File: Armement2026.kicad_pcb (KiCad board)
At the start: 2 copper layers, 87.5 x 61.5 mm, 24 parts, among them J1 Screw_Terminal_01x02, J10 Screw_Terminal_01x02, J11 Screw_Terminal_01x02, J12 Screw_Terminal_01x02, J2 Screw_Terminal_01x02, J5 Screw_Terminal_01x02, J6 Screw_Terminal_01x02, J8 Screw_Terminal_01x02, J9 Screw_Terminal_01x02, Q1 NTR4101PT1G, Q2 NTR4101PT1G, SW1 SW_Nidec_CAS-120A1, SW2 SW_Nidec_CAS-120A1, SW3 SW_Nidec_CAS-120A1, U1 LDO_4v2-MIC5209-4.2YS-TR

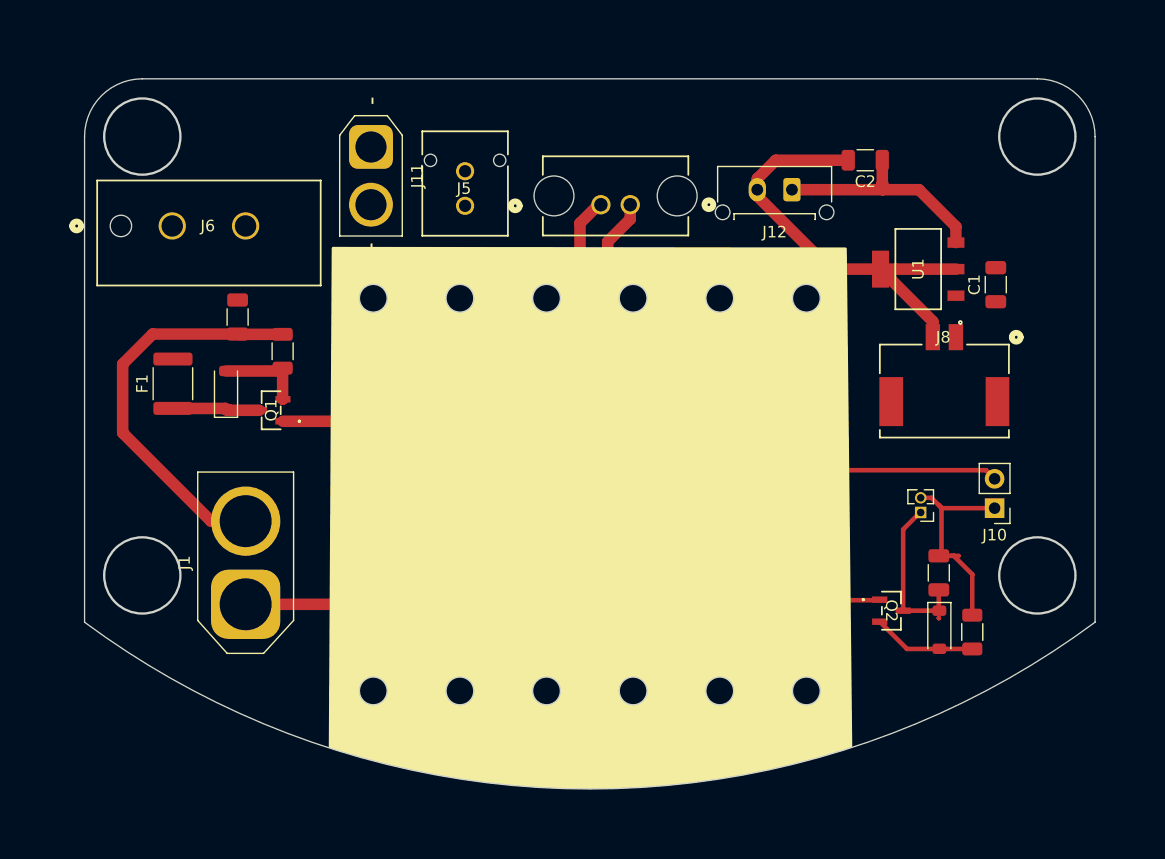
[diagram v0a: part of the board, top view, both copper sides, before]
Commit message: PCB Armement IRECxFAR-OUT
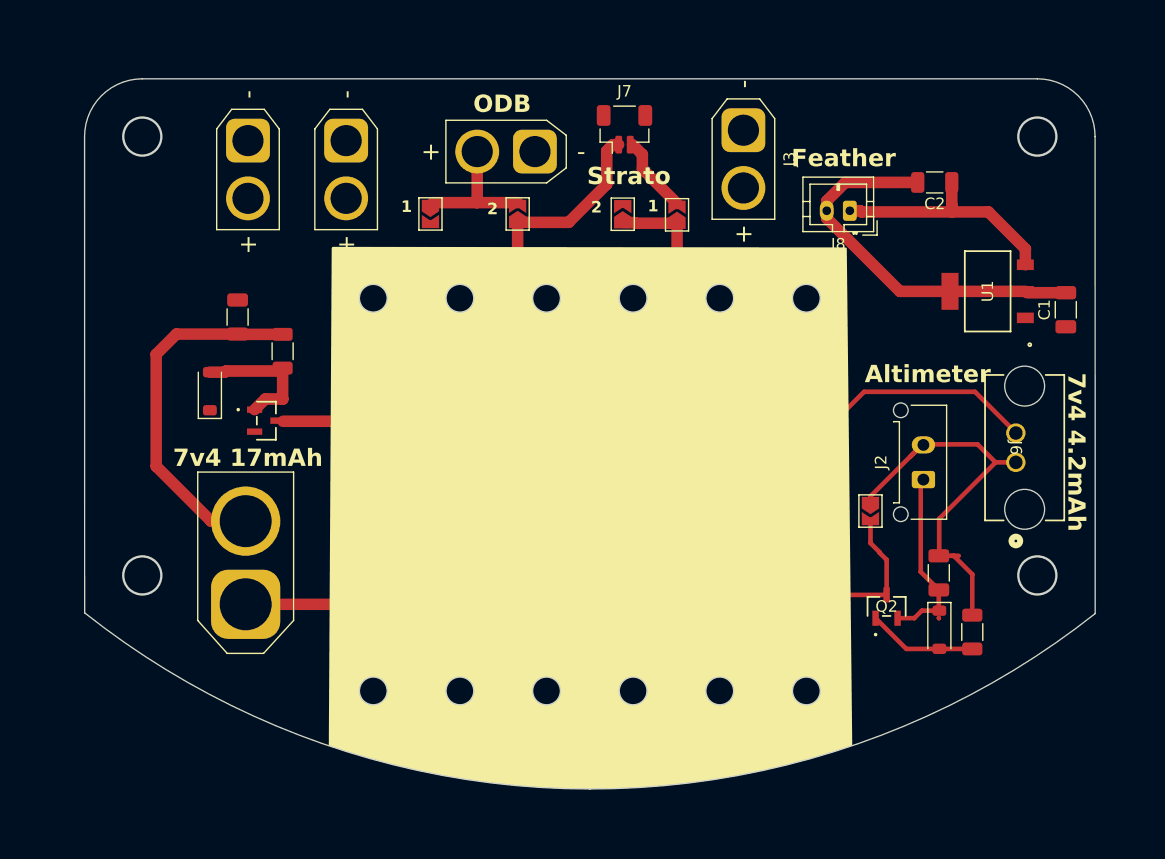
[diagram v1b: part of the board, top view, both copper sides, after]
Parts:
- removed F1: Polyfuse, Fuse:Fuse_1812_4532Metric
- removed J10: Screw_Terminal_01x02, Connector_PinHeader_2.54mm:PinHeader_1x02_P2.54mm_Vertical
- removed J12: Screw_Terminal_01x02, Connector_Molex:Molex_Micro-Fit_3.0_43650-0215_1x02_P3.00mm_Vertical
- removed J9: Screw_Terminal_01x02, Connector_PinHeader_1.27mm:PinHeader_1x02_P1.27mm_Vertical
- added J3: Screw_Terminal_01x02, Connector_AMASS:AMASS_XT30U-M_1x02_P5.0mm_Vertical, F.Cu at (113.0, 104.5)
- added J4: Screw_Terminal_01x02, Connector_AMASS:AMASS_XT30U-M_1x02_P5.0mm_Vertical, F.Cu at (70.2, 105.3)
- added J7: Screw_Terminal_01x02, Connector_JST:JST_SH_BM02B-SRSS-TB_1x02-1MP_P1.00mm_Vertical, F.Cu at (102.8, 104.4)
- added JP1: SolderJumper_2_Open, Jumper:SolderJumper-2_P1.3mm_Open_TrianglePad1.0x1.5mm, F.Cu at (124.0, 137.4)
- added JP2: SolderJumper_2_Open, Jumper:SolderJumper-2_P1.3mm_Open_TrianglePad1.0x1.5mm, F.Cu at (86.0, 111.7)
- added JP3: SolderJumper_2_Open, Jumper:SolderJumper-2_P1.3mm_Open_TrianglePad1.0x1.5mm, F.Cu at (102.6, 111.7)
- added JP4: SolderJumper_2_Open, Jumper:SolderJumper-2_P1.3mm_Open_TrianglePad1.0x1.5mm, F.Cu at (107.3, 111.8)
- added JP5: SolderJumper_2_Open, Jumper:SolderJumper-2_P1.3mm_Open_TrianglePad1.0x1.5mm, F.Cu at (93.5, 111.7)
- J2: footprint footprints:CONN_70545-xxxx_02_MOL -> Connector_Molex:Molex_Micro-Fit_3.0_43650-0215_1x02_P3.00mm_Vertical
- J5: footprint 3mm header 2x1:CONN_SD-44067-001_02_MOL -> Connector_AMASS:AMASS_XT30U-M_1x02_P5.0mm_Vertical
- J6: footprint footprints:CONN_SDA_43255-00XX_02_MOL -> footprints:CONN_70545-xxxx_02_MOL
- J8: footprint footprints:CONN02_560020_MOL -> Connector_JST:JST_PH_B2B-PH-K_1x02_P2.00mm_Vertical
- moved J6 75.9 mm to (136.6, 133.2), turned to -90 degrees
- moved J2 34.8 mm to (128.6, 134.7), turned to 90 degrees
- moved J8 17.6 mm to (122.3, 111.4), turned to 180 degrees
- moved J5 7.66 mm to (95.0, 106.3), turned to 180 degrees
- moved C1 6.44 mm to (141.0, 120.0)
- moved C2 6.31 mm to (129.6, 109.0)
- moved U1 6.31 mm to (134.2, 118.4)
- moved J11 2.22 mm to (78.7, 105.3)
- moved DZ1 1.40 mm to (66.8, 127.0)
- moved Q1 0.99 mm to (71.7, 129.6), turned to -90 degrees
- moved Q2 0.56 mm to (125.4, 145.7), turned to 0 degrees
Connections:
- C2 pad 1: Net-(J12-Pin_1) -> Net-(J8-Pin_1)
- C7 pad 2: Net-(J10-Pin_1) -> Net-(J2-Pin_2)
- DZ1 pad 1: Net-(DZ1-K) -> 7v4
- J1 pad 1: GND -> Net-(J1-Pin_1)
- J2 pad 1: Net-(J2-Pin_1) -> Net-(DZ2-K)
- J5 pad 1: 7v4 -> GND
- J5 pad 2: GND -> Net-(J5-Pin_2)
- J6 pad 1: 7v4 -> Net-(J2-Pin_2)
- J6 pad 2: GND -> Net-(J6-Pin_2)
- J8 pad 1: 7v4 -> Net-(J8-Pin_1)
- PWR_R2 pad 2: Net-(J10-Pin_1) -> Net-(J2-Pin_2)
- Q1 pad 1: GND -> Net-(Q1-D)
- Q1 pad 3: Net-(DZ1-K) -> 7v4
- SW1 pad 1: GND -> Net-(J1-Pin_1)
- SW1 pad 2: GND -> Net-(Q1-D)
- SW2 pad 1: Net-(J2-Pin_1) -> Net-(J7-Pin_1)
- SW2 pad 2: Net-(J2-Pin_2) -> Net-(JP3-A)
- SW3 pad 2: Net-(J10-Pin_2) -> Net-(J6-Pin_2)
- U1 pad 3: Net-(J12-Pin_1) -> Net-(J8-Pin_1)
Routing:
- net Net-(J7-Pin_1): track 0.00 -> 48.6 mm
- net Net-(J2-Pin_1): track 38.3 -> 0.00 mm
- net GND: track 101.7 -> 64.1 mm
- net Net-(JP3-A): track 0.00 -> 31.7 mm
- net Net-(J6-Pin_2): track 0.00 -> 27.7 mm
- net Net-(J10-Pin_2): track 21.9 -> 0.00 mm
- net Net-(J8-Pin_1): track 0.00 -> 20.5 mm
- net Net-(J12-Pin_1): track 19.5 -> 0.00 mm
- net Net-(J10-Pin_1): track 18.9 -> 0.00 mm
- net Net-(J1-Pin_1): track 0.00 -> 14.8 mm
- net Net-(Q1-D): track 0.00 -> 14.5 mm
- net Net-(J5-Pin_2): track 0.00 -> 13.4 mm
- net Net-(JP1-B): track 10.5 -> 18.3 mm
- net Net-(DZ1-K): track 7.56 -> 0.00 mm
- net Net-(J7-Pin_2): track 0.00 -> 6.69 mm
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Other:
- outline, holes or cut-outs redrawn
- board text added: "1"
- board text added: "2"
- board text added: "7v4 17mAh"
- board text added: "7v4 4.2mAh"
- board text added: "Altimeter"
- board text added: "Feather"
- board text added: "ODB"
- board text added: "Option 1: Solder this option to use the ODB as the third flight computer. Option 2: Solder this option to use the ODB as the second flight computer (without the Stratologger)."
- board text added: "PCB Armement 2026 IREC + Far-Out Alexis Giroux"
- board text added: "Strato"
